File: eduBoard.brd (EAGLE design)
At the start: 101.6 x 53.3 mm, 63 parts, among them IC1 NCP1117ST50T3G, IC3 ATMEGA2560-16AU, IC4 ATMEGA16U2-MU, IC6 LP2985-33DBVR, IC7 LMV358IDGKR, T1 FDN340P, X1 POWERSUPPLY_DC21MMX, X2 USB-B_TH, Y1 CSTCE16M0V53-R0 16MHZ, Y2 16MHz

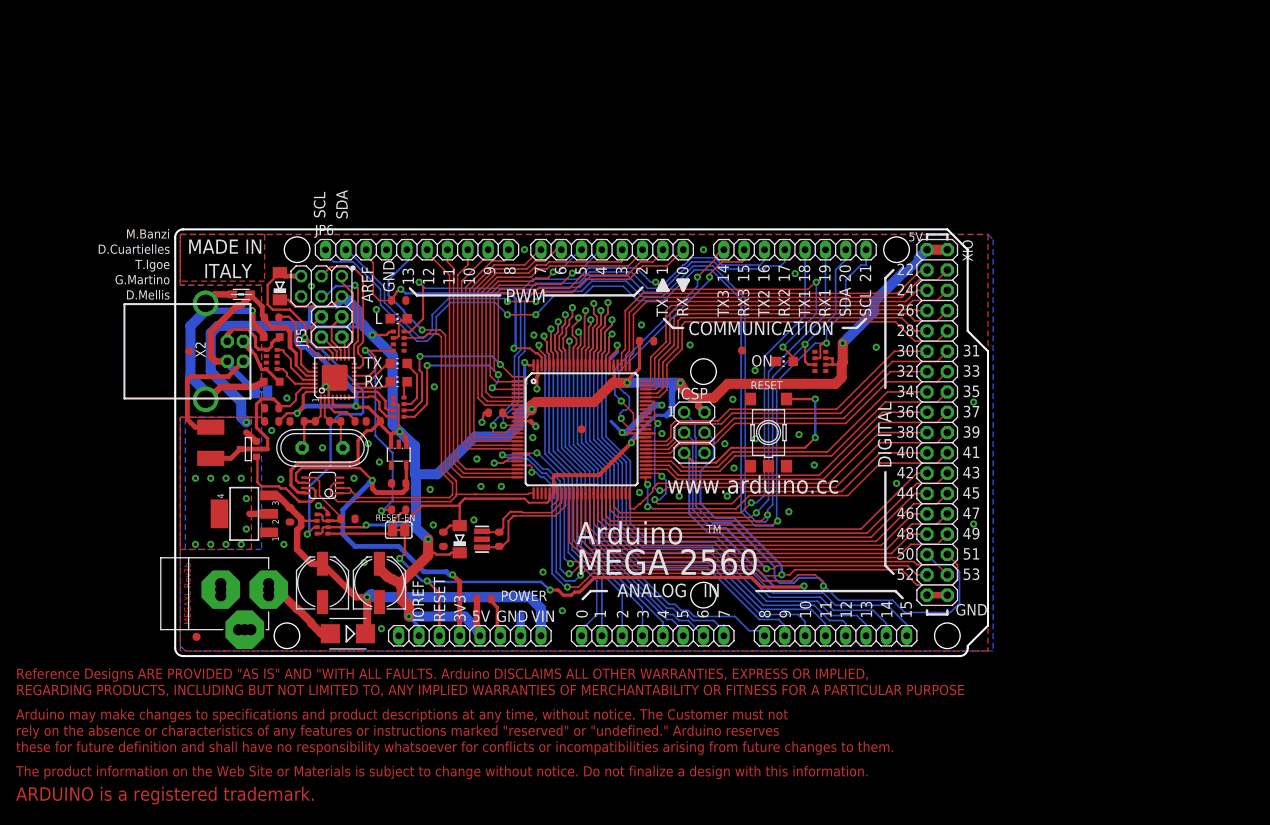
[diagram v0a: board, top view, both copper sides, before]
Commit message: nicer mega shield
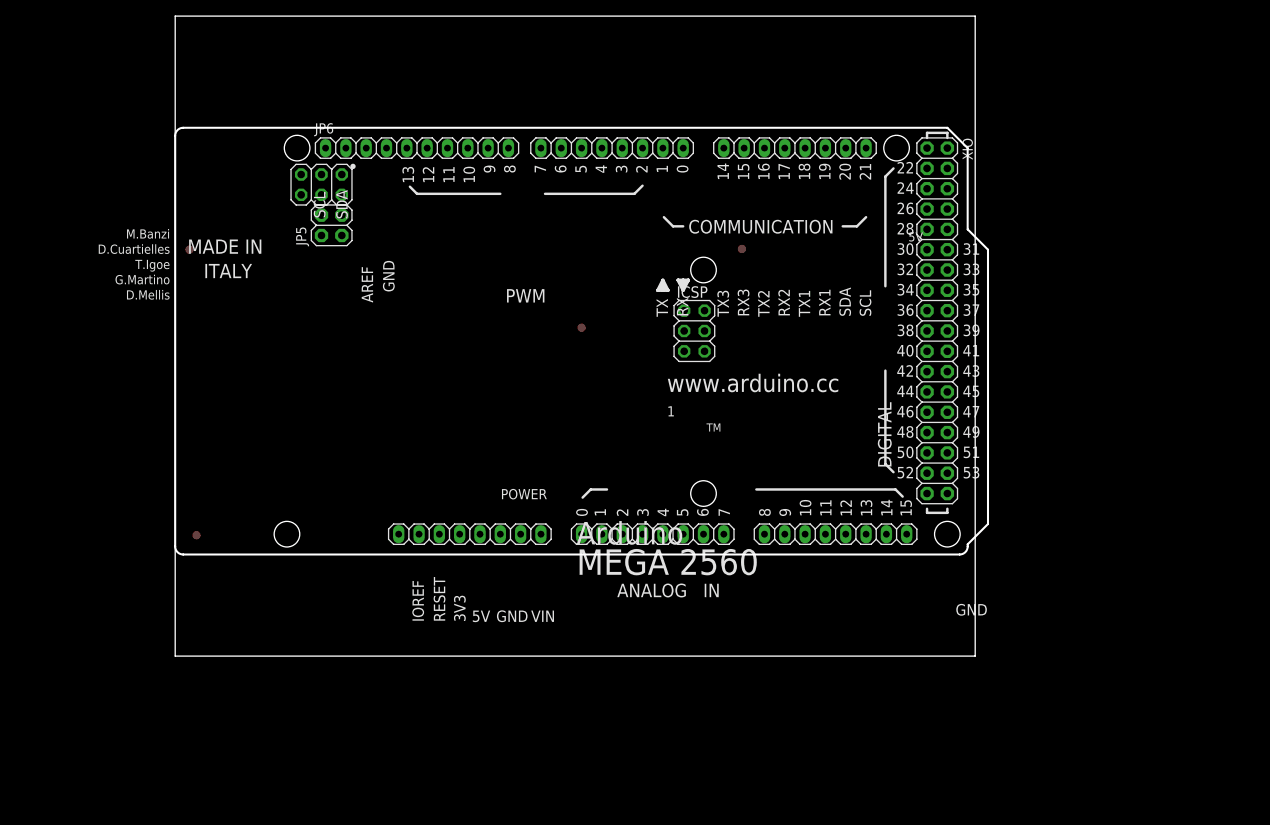
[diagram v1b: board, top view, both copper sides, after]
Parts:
- removed C1, C14, C15: 22p, SmartPrj:C0603-ROUND
- removed C10, C13: 1u, SmartPrj:C0603-ROUND
- removed C11, C12, C2, C3, C4, C5, C6, C7, C8, C9: 100n, SmartPrj:C0603-ROUND
- removed D1: M7, diode:SMB
- removed D2, D3: CD1206-S01575, diode:MINIMELF
- removed F1: MF-MSMF050-2 500mA, rcl:L1812
- removed GROUND, RESET-EN: (no value), jumper:SJ
- removed IC1: NCP1117ST50T3G, linear:SOT223
- removed IC3: ATMEGA2560-16AU, SmartPrj:TQFP100
- removed IC4: ATMEGA16U2-MU, SmartPrj:MLF32
- removed IC6: LP2985-33DBVR, SmartPrj:SOT23-DBV
- removed IC7: LMV358IDGKR, linear:MSOP08
- removed L, RX, TX: YELLOW, led:CHIP-LED0805
- removed L1: BLM21, wuerth-elektronik:0805
- removed ON: GREEN, led:CHIP-LED0805
- removed PC1, PC2: 47u, rcl:PANASONIC_D
- removed R1, R2: 1M, SmartPrj:R0603-ROUND
- removed RESET: TS42031-160R-TR-7260, SmartPrj:TS42
- removed RN1, RN5: 10K, resistor-dil:CAT16
- removed RN2: 22R, resistor-dil:CAY16
- removed RN3, RN4: 1k, resistor-dil:CAY16
- removed T1: FDN340P, zetex:SOT-23
- removed U$1: DISCLAIMER, SmartPrj:DISCLAIMER
- removed X1: POWERSUPPLY_DC21MMX, SmartPrj:POWERSUPPLY_DC-21MM
- removed X2: USB-B_TH, SmartPrj:PN61729
- removed Y1: CSTCE16M0V53-R0 16MHZ, SmartPrj:RESONATOR
- removed Y2: 16MHz, SmartPrj:QS
- removed Z1, Z2: CG0603MLC-05E, varistor:CT/CN0603
- moved COMMUNICATION 12.7 mm to (77.5, 63.5)
- moved FD1 12.7 mm to (70.8, 50.9)
- moved JP6 12.7 mm to (30.2, 63.5)
- moved PWML 12.7 mm to (54.6, 63.5)
- moved ADCH 12.7 mm to (82.5, 15.2)
- moved ADCL 12.7 mm to (59.7, 15.2)
- moved FD2 12.7 mm to (2.67, 15.1)
- moved FD4 12.7 mm to (50.8, 41.0)
- moved ICSP 12.7 mm to (64.9, 40.6)
- moved POWER 12.7 mm to (36.8, 15.2)
- moved FD3 12.7 mm to (1.78, 50.8)
- moved ICSP1 12.7 mm to (18.3, 58.9)
- moved JP5 12.7 mm to (19.6, 53.8)
- moved XIO 12.7 mm to (95.2, 41.9)
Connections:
- removed net 5-GND: RESET.5
- removed net CMP: C12.2, IC7.5, RN5.3, RN5.5
- removed net D+: RN2.5, X2.3, Z2.2
- removed net D-: RN2.8, X2.2, Z1.2
- removed net DTR: C7.1, IC4.13, RN3.4
- removed net GATE_CMD: IC7.7, T1.3
- removed net L13: IC7.1, IC7.2, RN3.7
- removed net M8RXD: IC4.9, RN4.7
- removed net M8TXD: IC4.8, RN4.8
- removed net N$2: L.A, RN3.2
- removed net N$54: RN4.4, RX.A
- removed net N$55: RN4.3, TX.A
- removed net PWRIN: D1.A, X1.2
- removed net RD+: IC4.29, RN2.4
- removed net RD-: IC4.30, RN2.1
- removed net RXL: IC4.10, RX.C
- removed net TXL: IC4.11, TX.C
- removed net UGND: C10.2, GROUND.1, IC4.28, L1.1, X2.4
- removed net USBVCC: C8.1, F1.1, IC4.31, T1.1
- removed net USHIELD: L1.2, X2.P$1, X2.P$2, Z1.1, Z2.1
- removed net VUCAP: C10.1, IC4.27
- removed net XT1: C14.1, IC4.1, R2.1, Y2.2
- removed net XT2: C15.1, IC4.2, R2.2, Y2.1
- removed net XTAL1: IC3.34, R1.1, Y1.3
- removed net XTAL2: IC3.33, R1.2, Y1.1
- removed net XVCC: F1.2, X2.1
- net +3V3: no longer C13.2, IC6.5, IC7.6
- net +5V: no longer C11.2, C4.1, C5.1, C6.1, C9.1, D2.C, D3.C, IC1.2, IC1.4, IC3.10, IC3.100, IC3.31, IC3.61, IC3.80, IC4.32, IC4.4, IC6.1, IC6.3, IC7.8, PC2.+, RN1.6, RN1.7, RN3.1, RN4.5, RN4.6, RN5.2, RN5.8, T1.2
- net 8PB4: no longer IC4.18
- net 8PB5: no longer IC4.19
- net 8PB6: no longer IC4.20
- net 8PB7: no longer IC4.21
- net ADC0: no longer IC3.97
- net ADC1: no longer IC3.96
- net ADC10: no longer IC3.87
- net ADC11: no longer IC3.86
- net ADC12: no longer IC3.85
- net ADC13: no longer IC3.84
- net ADC14: no longer IC3.83
- net ADC15: no longer IC3.82
- net ADC2: no longer IC3.95
- net ADC3: no longer IC3.94
- net ADC4: no longer IC3.93
- net ADC5: no longer IC3.92
- net ADC6: no longer IC3.91
- net ADC7: no longer IC3.90
- net ADC8: no longer IC3.89
- net ADC9: no longer IC3.88
- net AREF: no longer C3.1, IC3.98
- net GND: no longer C1.2, C11.1, C12.1, C13.1, C14.2, C15.2, C2.2, C3.2, C4.2, C5.2, C6.2, C8.2, C9.2, GROUND.2, IC1.1, IC3.11, IC3.32, IC3.62, IC3.81, IC3.99, IC4.3, IC4.33, IC6.2, IC7.4, L.C, ON.C, PC1.-, PC2.-, RESET.1, RESET.2, RN3.5, RN5.4, X1.1, X1.3, Y1.2
- net MISO2: no longer IC4.17
- net MOSI2: no longer IC4.16
- net N$3: now also JP6.2; no longer ON.A, RN3.8
- net PA0: no longer IC3.78
- net PA1: no longer IC3.77
- net PA2: no longer IC3.76
- net PA3: no longer IC3.75
- net PA4: no longer IC3.74
- net PA5: no longer IC3.73
- net PA6: no longer IC3.72
- net PA7: no longer IC3.71
- net PB0: no longer IC3.19
- net PB1: no longer IC3.20
- net PB2: no longer IC3.21
- net PB3: no longer IC3.22
- net PB4: no longer IC3.23
- net PB5: no longer IC3.24
- net PB6: no longer IC3.25
- net PB7: no longer IC3.26, IC7.3
- net PC0: no longer IC3.53
- net PC1: no longer IC3.54
- net PC2: no longer IC3.55
- net PC3: no longer IC3.56
- net PC4: no longer IC3.57
- net PC5: no longer IC3.58
- net PC6: no longer IC3.59
- net PC7: no longer IC3.60
- net PD7: no longer IC3.50
- net PE0: no longer IC3.2, RN4.2
- net PE1: no longer IC3.3, RN4.1
- net PE3: no longer IC3.5
- net PE4: no longer IC3.6
- net PE5: no longer IC3.7
- net PG0: no longer IC3.51
- net PG1: no longer IC3.52
- net PG2: no longer IC3.70
- net PG5: no longer IC3.1
- net PH3: no longer IC3.15
- net PH4: no longer IC3.16
- net PH5: no longer IC3.17
- net PH6: no longer IC3.18
- net PL0: no longer IC3.35
- net PL1: no longer IC3.36
- net PL2: no longer IC3.37
- net PL3: no longer IC3.38
- net PL4: no longer IC3.39
- net PL5: no longer IC3.40
- net PL6: no longer IC3.41
- net PL7: no longer IC3.42
- net RESET: now also POWER.1; no longer C1.1, C7.2, D3.A, IC3.30, POWER.3, RESET-EN.1, RESET-EN.2, RESET.3, RESET.4, RN5.1
- net RESET2: no longer D2.A, IC4.24, RN5.7
- net RXD1: no longer IC3.45
- net RXD2: no longer IC3.12
- net RXD3: no longer IC3.63
- net SCK2: no longer IC4.15
- net SCL: no longer IC3.43, RN1.2
- net SDA: no longer IC3.44, JP6.2, RN1.3
- net TXD1: no longer IC3.46
- net TXD2: no longer IC3.13
- net TXD3: no longer IC3.64
- net VIN: no longer C2.1, D1.C, IC1.3, PC1.+, RN5.6
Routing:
- net +5V: track 345.6 -> 0.00 mm, vias 24 -> 0
- net SCL: track 167.8 -> 0.00 mm, vias 4 -> 0
- net SDA: track 158.9 -> 0.00 mm, vias 4 -> 0
- net RESET: track 158.1 -> 0.00 mm, vias 6 -> 0
- net PB3: track 115.4 -> 0.00 mm, vias 3 -> 0
- net PB2: track 104.5 -> 0.00 mm, vias 3 -> 0
- net PB1: track 91.3 -> 0.00 mm, vias 3 -> 0
- net ADC13: track 75.2 -> 0.00 mm, vias 1 -> 0
- net ADC14: track 72.8 -> 0.00 mm, vias 1 -> 0
- net N$3: track 72.5 -> 0.00 mm, vias 4 -> 0
- net ADC11: track 71.2 -> 0.00 mm, vias 1 -> 0
- net ADC12: track 71.0 -> 0.00 mm, vias 1 -> 0
- net ADC15: track 70.6 -> 0.00 mm, vias 1 -> 0
- net PB0: track 66.4 -> 0.00 mm, vias 2 -> 0
- net PB7: track 65.1 -> 0.00 mm, vias 1 -> 0
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- removed copper zone on layer 1, net +5V
- removed copper zone on layer 16, net +5V
- removed copper zone on layer 1, net GND
- removed copper zone on layer 16, net GND
- removed copper zone on layer 1, net N$1
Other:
- board size 101.6 x 53.3 mm -> 101.6 x 80 mm
- board text removed: "L"
- board text removed: "MEGAXL-Rev3b"
- board text removed: "ON"
- board text removed: "PC1"
- board text removed: "PC2"
